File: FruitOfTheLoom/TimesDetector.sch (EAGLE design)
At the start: 2 parts

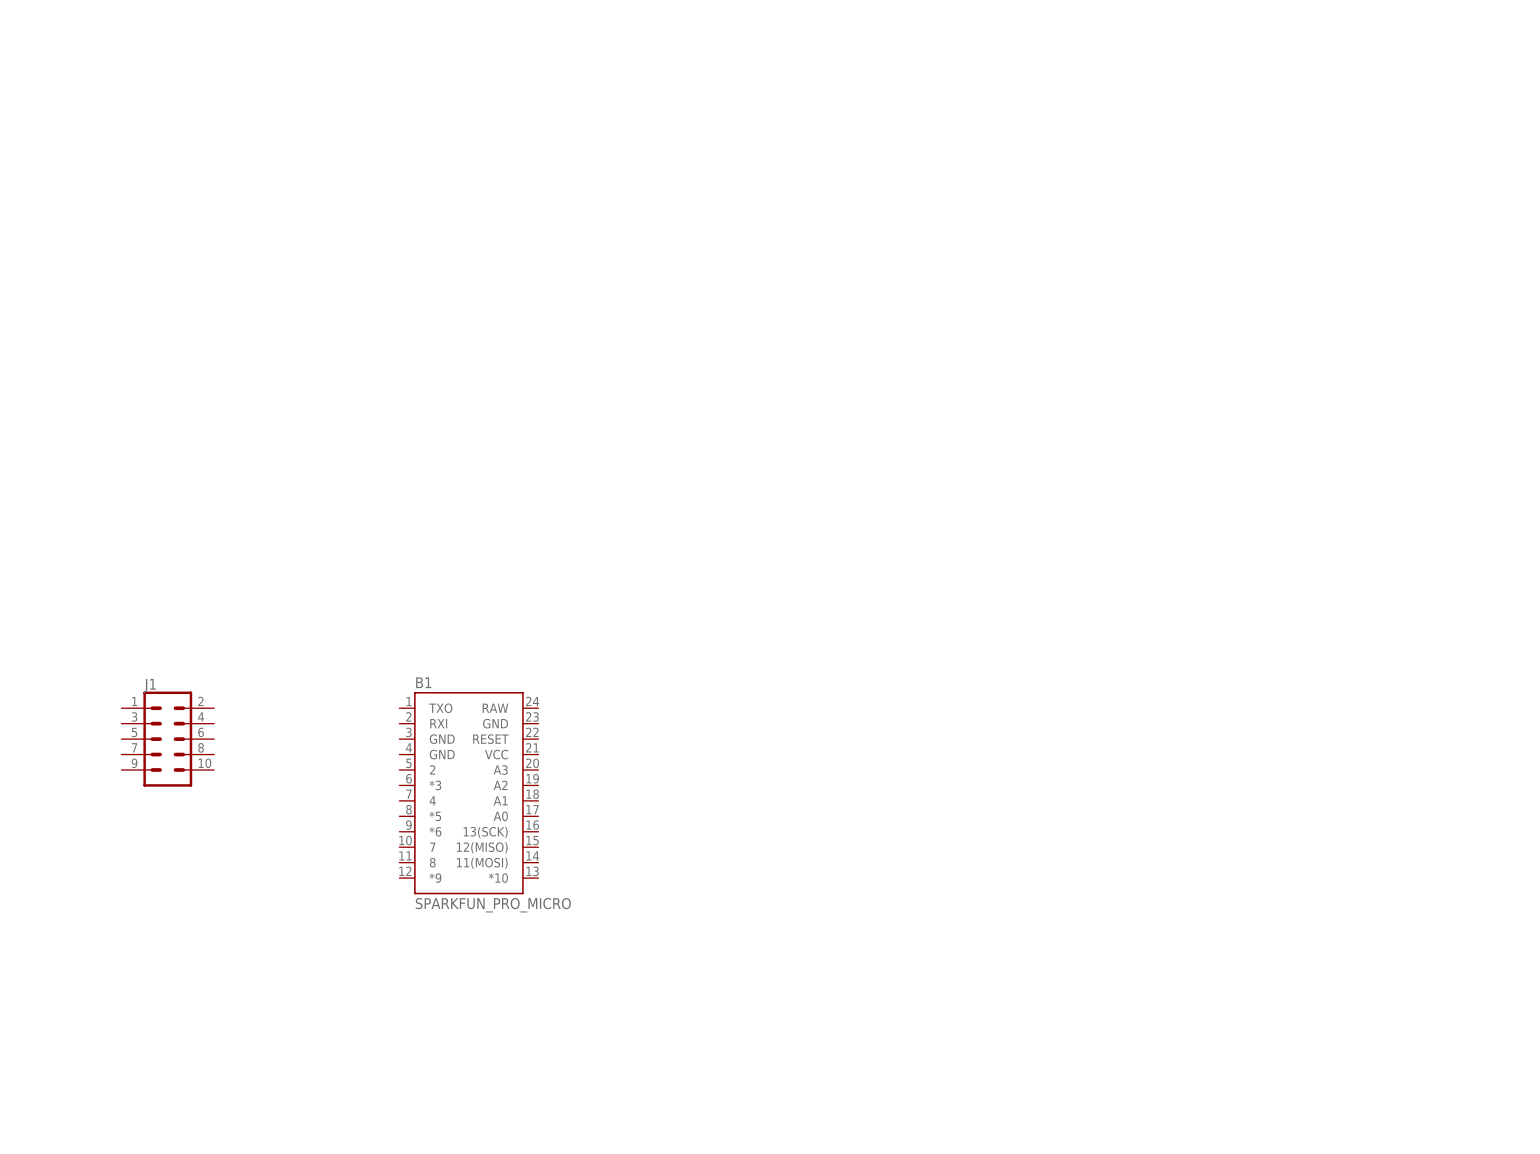
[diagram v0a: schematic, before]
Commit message: ordenamiento y conexion
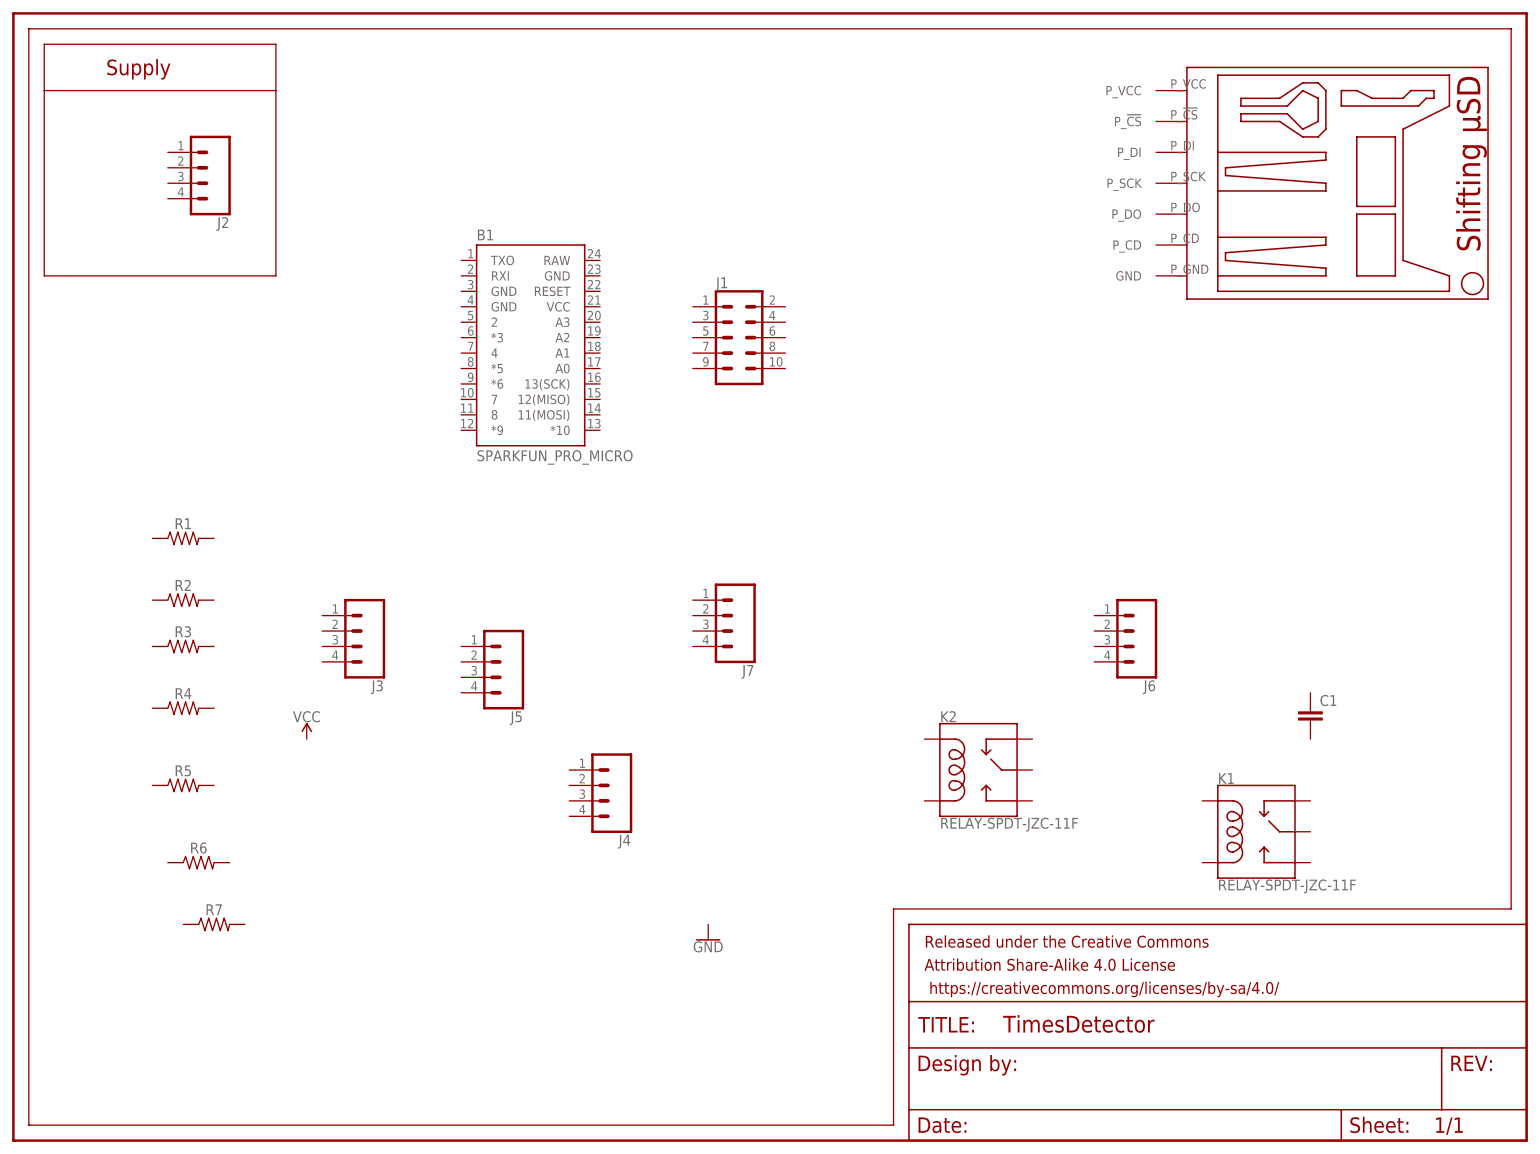
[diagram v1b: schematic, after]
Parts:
- added C1: (no value), capacitor-wima:C10/6
- added FRAME1: FRAME-LETTER, SparkFun-Aesthetics:FRAME-LETTER
- added J2, J3, J4, J5, J6, J7: (no value), SparkFun-Connectors:CONN_04POLAR
- added K1, K2: RELAY-SPDT-JZC-11F, SparkFun-Electromechanical:RELAY-SPDT-JZC-11F
- added MODULE1: MICROSD_SPARKFUN_LEVEL_SHIFTING_MODULE, MODULOS_MICROSD:MICROSD_SPARKFUN_LEVEL_SHIFTING_MODULE
- added R1, R2, R3, R4, R5, R6, R7: (no value), SparkFun-Resistors:RESISTORAXIAL-0.3
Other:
- note added: "Supply"
- moved on the sheet: B1, J1
